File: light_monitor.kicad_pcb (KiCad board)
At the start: 2 copper layers, 32.9 x 32.9 mm, 35 parts, among them IC1 TSL25911FN, J3 USB_B_Micro, U1 STM32L432KCUx, U2 STDC14, U3 TPS610986, U4 LDK130PU33R_DFN6, U5 RV-8803-C7, X1 board_lens

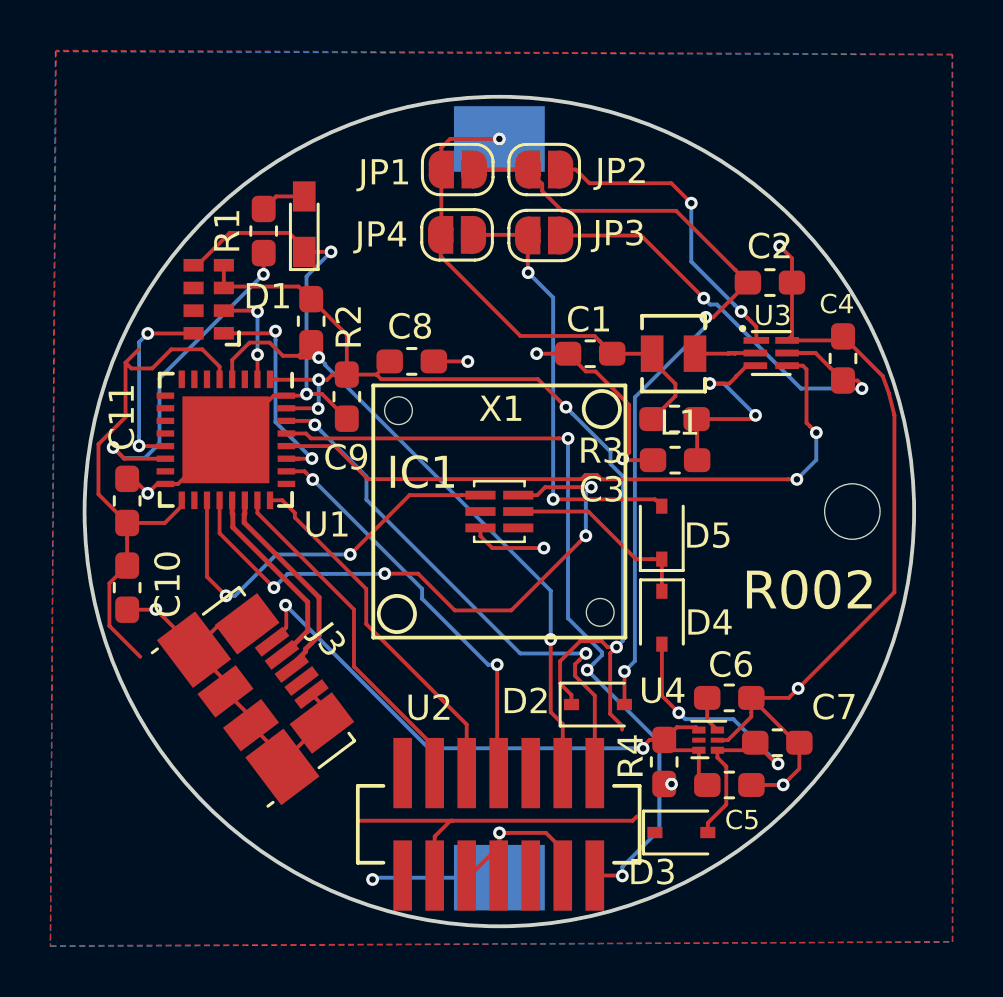
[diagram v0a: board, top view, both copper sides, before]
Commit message: sensor complete
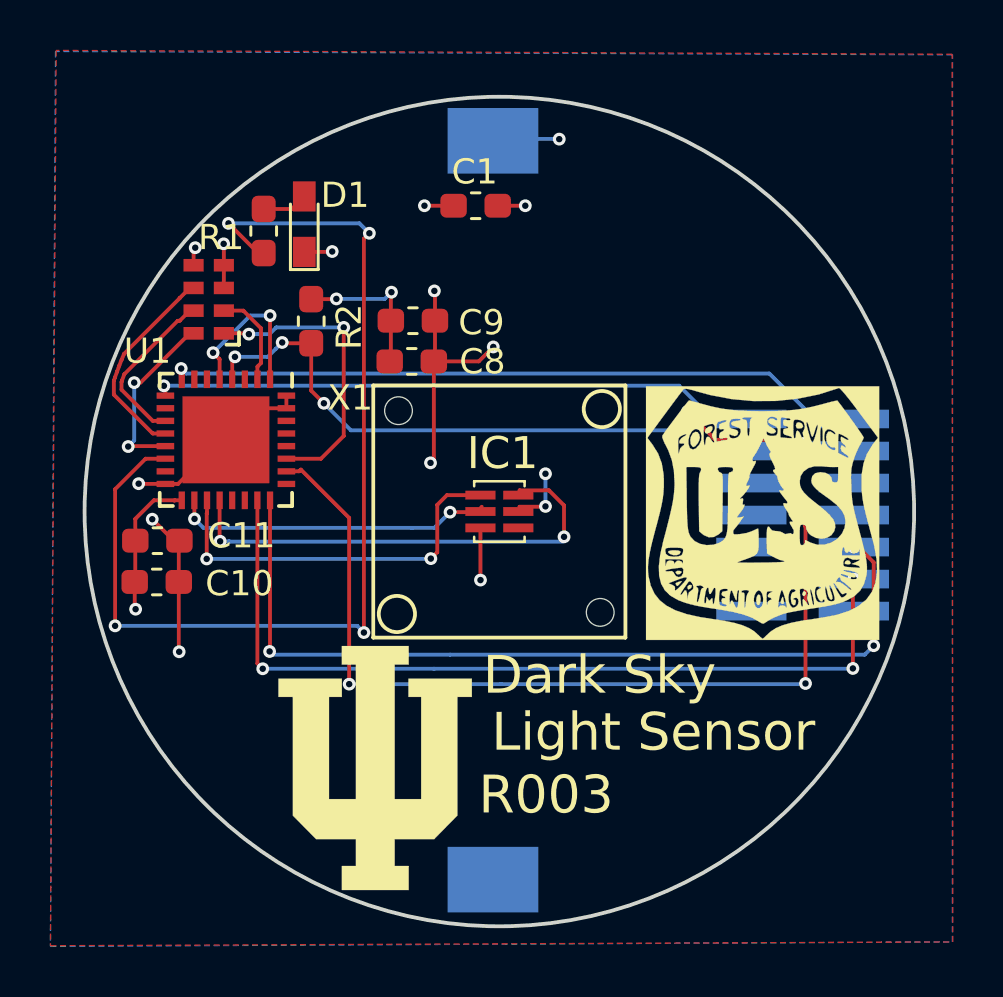
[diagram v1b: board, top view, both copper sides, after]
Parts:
- removed C2, C5: 10uF, Capacitor_SMD:C_0603_1608Metric_Pad1.05x0.95mm_HandSolder
- removed C3: 0.1uF, Capacitor_SMD:C_0603_1608Metric_Pad1.05x0.95mm_HandSolder
- removed C4, C7: 1uF, Capacitor_SMD:C_0603_1608Metric_Pad1.05x0.95mm_HandSolder
- removed C6: 10nF, Capacitor_SMD:C_0603_1608Metric_Pad1.05x0.95mm_HandSolder
- removed D2, D3, D4, D5: D_Schottky, Diode_SMD:D_SOD-323
- removed H1: MountingHole, MountingHole:MountingHole_2.2mm_M2
- removed J3: USB_B_Micro, Connector_USB:USB_Micro-B_Molex_47346-0001
- removed JP1, JP2, JP3, JP4: Jumper_2_Open, Jumper:SolderJumper-2_P1.3mm_Open_RoundedPad1.0x1.5mm
- removed L1: 4.7uH, bhimebau_inductor:TDKVLF3025
- removed R3: 400, Resistor_SMD:R_0603_1608Metric_Pad1.05x0.95mm_HandSolder
- removed R4: 100k, Resistor_SMD:R_0603_1608Metric_Pad1.05x0.95mm_HandSolder
- removed U3: TPS610986, SON50P150X150X80-6N:SON50P150X150X80-6N
- removed U4: LDK130PU33R_DFN6, Package_DFN_QFN:DFN-6_1.3x1.2mm_P0.4mm
- added G***: LOGO, boardlogo:us_forest_service_logo, F.Cu at (123.8, 105.3)
- added G***: LOGO, boardlogo:board_logo, F.Cu at (108.4, 115.4)
- U2: moved to B.Cu
- moved U2 17.2 mm to (125.4, 105.4), turned to 90 degrees
- moved C1 7.42 mm to (112.4, 93.1)
- moved C9 3.99 mm to (109.9, 97.7), turned to 0 degrees
- moved C11 1.98 mm to (99.8, 106.4), turned to 0 degrees
- moved C10 1.19 mm to (99.8, 108.0), turned to 0 degrees
- moved BT1 0.27 mm to (113.1, 105.2)
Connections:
- BT1 pad 1: /VBATT -> VDD
- C1 pad 1: /VBATT -> VDD
- IC1 pad 2: Net-(IC1-Pad2) -> /sensor_int
- IC1 pad 4: Net-(IC1-Pad4) -> (no net)
- IC1 pad 5: +VSW -> VDD
- U1 pad 10: Net-(U1-Pad10) -> (no net)
- U1 pad 11: Net-(U1-Pad11) -> /rtc_EVI
- U1 pad 12: Net-(U1-Pad12) -> /rtc_nINT
- U1 pad 15: Net-(U1-Pad15) -> (no net)
- U1 pad 18: Net-(U1-Pad18) -> /sensor_int
- U1 pad 21: /USB_N -> (no net)
- U1 pad 22: /USB_P -> (no net)
- U1 pad 25: Net-(U1-Pad25) -> (no net)
- U1 pad 28: /SW_MODE -> (no net)
- U1 pad 29: /TX -> (no net)
- U1 pad 3: Net-(U1-Pad3) -> (no net)
- U1 pad 30: /RX -> (no net)
- U1 pad 31: VDD -> GND
- U1 pad 6: Net-(U1-Pad6) -> (no net)
- U1 pad 7: Net-(U1-Pad7) -> (no net)
- U1 pad 8: Net-(U1-Pad8) -> /TX
- U1 pad 9: Net-(U1-Pad9) -> /RX
- U2 pad 1: Net-(U2-Pad1) -> (no net)
- U2 pad 10: Net-(U2-Pad10) -> (no net)
- U2 pad 13: /TX -> /RX
- U2 pad 14: /RX -> /TX
- U2 pad 2: Net-(U2-Pad2) -> (no net)
- U2 pad 9: Net-(U2-Pad9) -> (no net)
- U5 pad 6: Net-(U5-Pad6) -> /rtc_nINT
- U5 pad 7: Net-(U5-Pad7) -> /rtc_EVI
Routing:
- net GND: track 99.7 -> 30.8 mm, vias 14 -> 10
- net VDD: track 77.9 -> 28.3 mm, vias 4 -> 11
- net +3V3: track 31.8 -> 0.00 mm, vias 2 -> 0
- net Net-(R1-Pad1): track 13.8 -> 41.5 mm, vias 2 -> 4
- net /SW_MODE: track 26.6 -> 0.00 mm, vias 2 -> 0
- net Net-(C5-Pad1): track 23.9 -> 0.00 mm, vias 2 -> 0
- net /SWO: track 16.1 -> 37.0 mm, vias 2 -> 3
- net /SWDCLK: track 14.3 -> 34.5 mm, vias 0 -> 3
- net /VBATT: track 20.1 -> 0.00 mm, vias 1 -> 0
- net /SWDIO: track 13.7 -> 33.7 mm, vias 0 -> 3
- net Net-(C4-Pad1): track 18.3 -> 0.00 mm, vias 2 -> 0
- net Net-(D5-Pad2): track 17.2 -> 0.00 mm, vias 2 -> 0
- net Net-(C7-Pad1): track 14.4 -> 0.00 mm, vias 2 -> 0
- net /sensor_int: track 0.00 -> 12.5 mm, vias 0 -> 2
- net Net-(JP2-Pad2): track 12.2 -> 0.00 mm, vias 2 -> 0
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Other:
- board text added: "Dark Sky"
- board text added: "Light Sensor"
- board text added: "R003"
- board text removed: "R002"
